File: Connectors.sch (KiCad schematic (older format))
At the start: 4 parts, among them J2 POWER_IN, J3 DBG_UART, J4 Conn_01x16

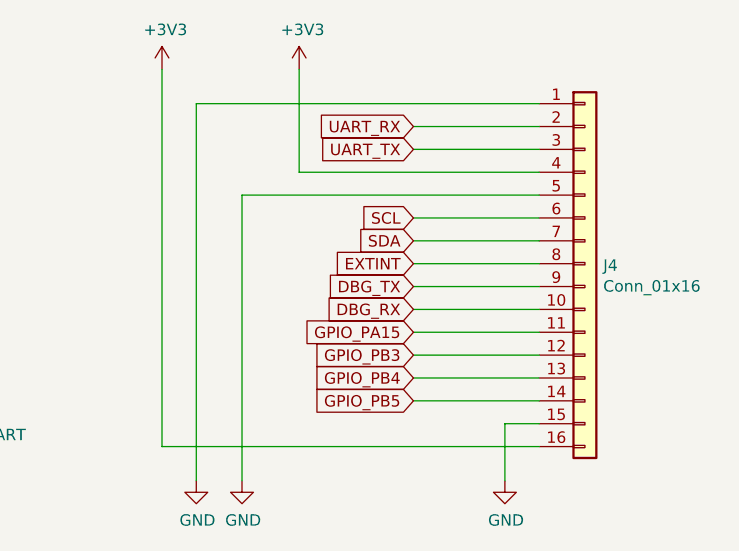
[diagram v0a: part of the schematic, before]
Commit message: many optimizations; LAYOUT!
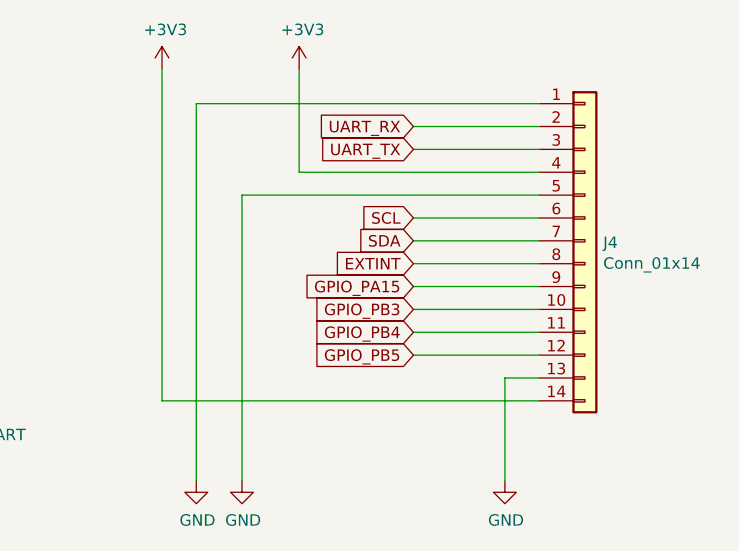
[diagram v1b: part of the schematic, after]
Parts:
- removed J4: Conn_01x16, Connector_PinHeader_2.54mm:PinHeader_1x16_P2.54mm_Vertical, symbol Connector_Generic:Conn_01x16
- added J4: Conn_01x14, Connector_PinHeader_2.54mm:PinHeader_1x14_P2.54mm_Vertical, symbol Connector_Generic:Conn_01x14
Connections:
- net +3V3: now also J4.14 (Pin_14), J4.4 (Pin_4)
- net EXTINT: now also J4.8 (Pin_8)
- net GND: now also J4.1 (Pin_1), J4.13 (Pin_13), J4.5 (Pin_5)
- net GPIO_PA15: now also J4.9 (Pin_9)
- net GPIO_PB3: now also J4.10 (Pin_10)
- net GPIO_PB4: now also J4.11 (Pin_11)
- net GPIO_PB5: now also J4.12 (Pin_12)
- net SCL: now also J4.6 (Pin_6)
- net SDA: now also J4.7 (Pin_7)
- net UART_RX: now also J4.2 (Pin_2)
- net UART_TX: now also J4.3 (Pin_3)
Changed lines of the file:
@@
 Text GLabel 9500 2250 0    50   Input ~ 0
 EXTINT
+Text GLabel 9500 2450 0    50   Input ~ 0
+GPIO_PB3
+Text GLabel 9500 2550 0    50   Input ~ 0
+GPIO_PB4
+Text GLabel 9500 2650 0    50   Input ~ 0
+GPIO_PB5
 Text GLabel 9500 2350 0    50   Input ~ 0
-DBG_TX
-Text GLabel 9500 2450 0    50   Input ~ 0
-DBG_RX
-Text GLabel 9500 2650 0    50   Input ~ 0
-GPIO_PB3
-Text GLabel 9500 2750 0    50   Input ~ 0
-GPIO_PB4
-Text GLabel 9500 2850 0    50   Input ~ 0
-GPIO_PB5
-Text GLabel 9500 2550 0    50   Input ~ 0
 GPIO_PA15
 $Comp
@@
 Wire Wire Line
 	10050 2250 9500 2250
-$Comp
-L Connector_Generic:Conn_01x16 J4
-U 1 1 5D1D5844
-P 10250 2250
-F 0 "J4" H 10330 2242 50  0000 L CNN
-F 1 "Conn_01x16" H 10330 2151 50  0000 L CNN
-F 2 "Connector_PinHeader_2.54mm:PinHeader_1x16_P2.54mm_Vertical" H 10250 2250 50  0001 C CNN
-F 3 "~" H 10250 2250 50  0001 C CNN
-	1    10250 2250
-	1    0    0    -1
-$EndComp
 Wire Wire Line
 	10050 2350 9500 2350
@@
 	9500 2450 10050 2450
 Wire Wire Line
-	10050 2550 9500 2550
+	9500 2550 10050 2550
 Wire Wire Line
 	9500 2650 10050 2650
-Wire Wire Line
-	9500 2750 10050 2750
-Wire Wire Line
-	9500 2850 10050 2850
 $Comp
 L Connector_Generic:Conn_01x03 J3
@@
 $EndComp
 Wire Wire Line
-	8400 1400 8400 3050
-Wire Wire Line
-	8400 3050 10050 3050
+	8400 1400 8400 2850
 $Comp
 L power:GND #PWR?
@@
 	1    0    0    -1
 $EndComp
-Wire Wire Line
-	9900 3200 9900 2950
-Wire Wire Line
-	9900 2950 10050 2950
 $Comp
 L power:+BATT #PWR0139
@@
 Wire Wire Line
 	8550 1550 10050 1550
+$Comp
+L Connector_Generic:Conn_01x14 J4
+U 1 1 5D1C10C6
+P 10250 2150
+F 0 "J4" H 10330 2142 50  0000 L CNN
+F 1 "Conn_01x14" H 10330 2051 50  0000 L CNN
+F 2 "Connector_PinHeader_2.54mm:PinHeader_1x14_P2.54mm_Vertical" H 10250 2150 50  0001 C CNN
+F 3 "~" H 10250 2150 50  0001 C CNN
+	1    10250 2150
+	1    0    0    -1
+$EndComp
+Wire Wire Line
+	10050 2750 9900 2750
+Wire Wire Line
+	10050 2850 8400 2850
+Wire Wire Line
+	9900 2750 9900 3200
 $EndSCHEMATC
